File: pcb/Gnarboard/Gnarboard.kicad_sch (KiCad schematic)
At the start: 2 parts, among them U2 MCP3208

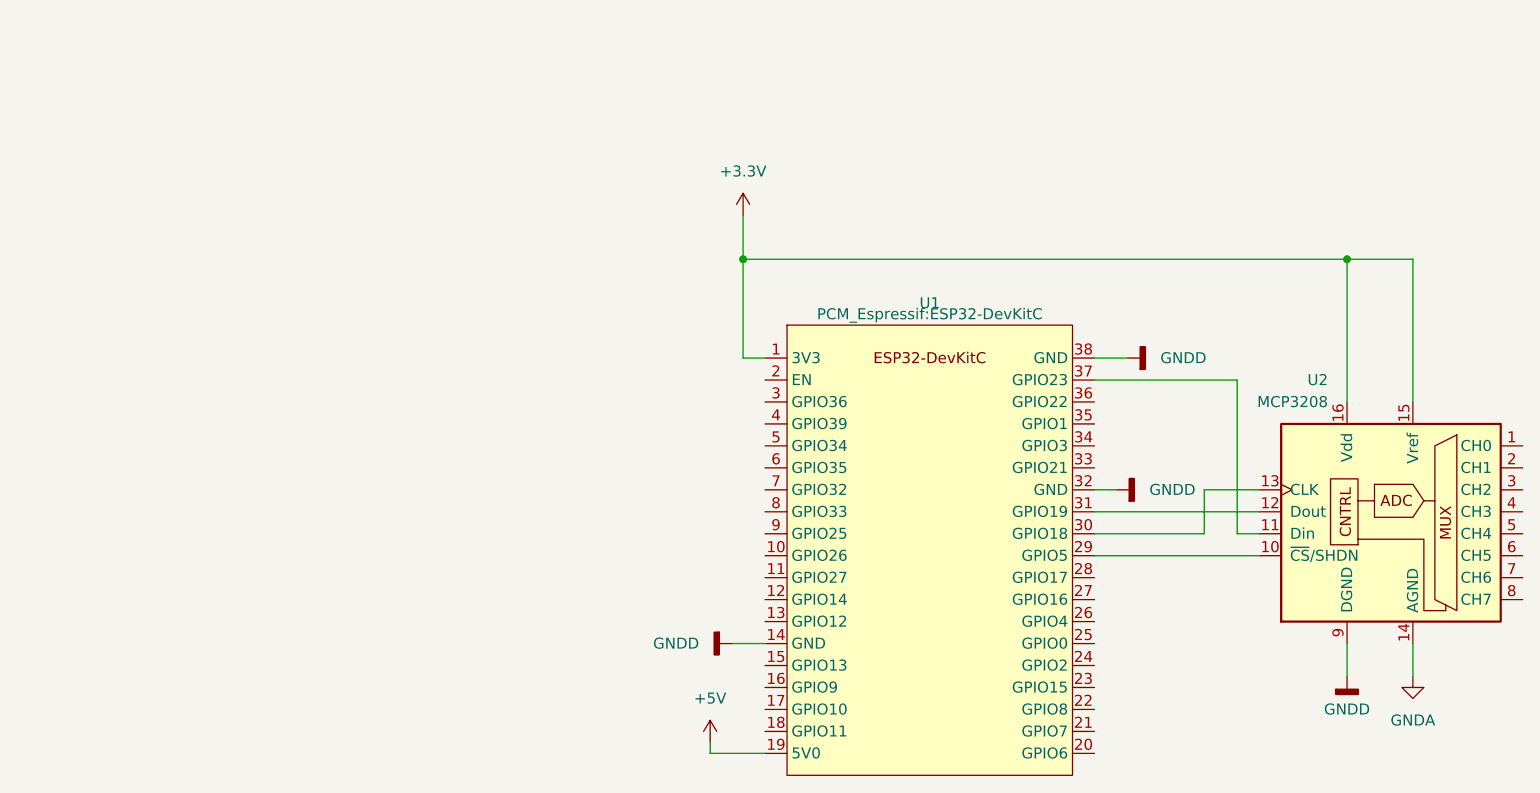
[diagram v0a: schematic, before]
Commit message: a bit more progress on the design. kicad pretty decent these days.
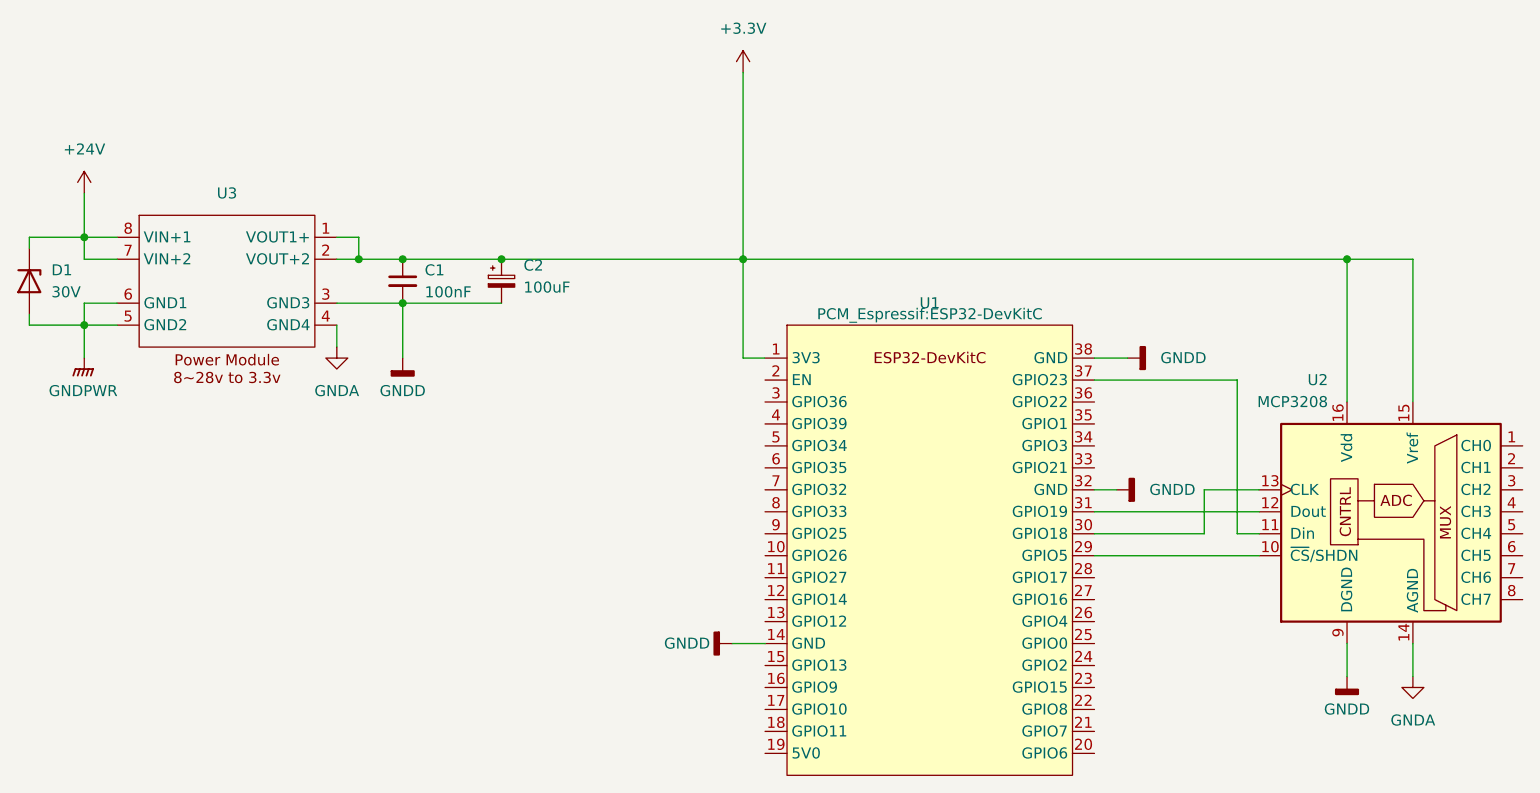
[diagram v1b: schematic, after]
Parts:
- added C1: 100nF, Capacitor_THT:C_Disc_D4.7mm_W2.5mm_P5.00mm, symbol Device:C_Small
- added C2: 100uF, Capacitor_THT:CP_Radial_D8.0mm_P5.00mm, symbol Device:C_Polarized_Small
- added D1: 30V, Diode_THT:D_DO-35_SOD27_P10.16mm_Horizontal, symbol Diode:ZPDxx
- added U3: ~, gnarboard:DF1768, symbol gnarboard:DFR0571
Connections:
- net +3.3V: now also C1.1, C2.1, U3.1 (VOUT1+), U3.2 (VOUT+2)
- net GNDA: now also U3.4 (GND4)
- net GNDD: now also C1.2, C2.2, U3.3 (GND3)
- net +5V: no longer names the net of U1.19 (5V0)
- new net +24V: D1.1 (K), U3.7 (VIN+2), U3.8 (VIN+1)
- new net GNDPWR: D1.2 (A), U3.5 (GND2), U3.6 (GND1)
